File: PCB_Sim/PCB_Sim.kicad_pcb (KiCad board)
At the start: 2 copper layers, 53.3 x 111.8 mm, 12 parts, among them J1 Maneuver_ICS, J2 Loadcell_front_1, J3 Loadcell_front_2, J4 Loadcell_back_1, J5 Loadcell_back_2, J6 Speaker, SW1 SW_DPST_x2, U1 Pico

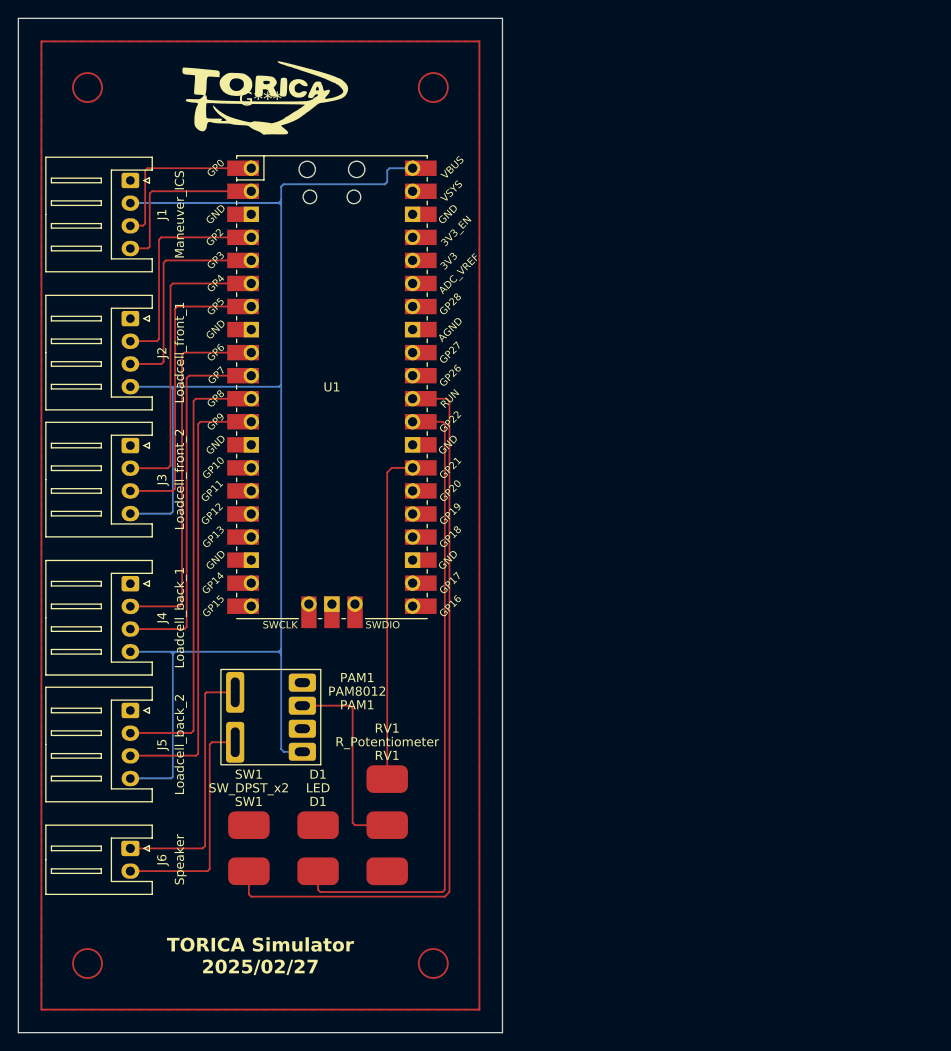
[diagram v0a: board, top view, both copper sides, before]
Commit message: ver.2
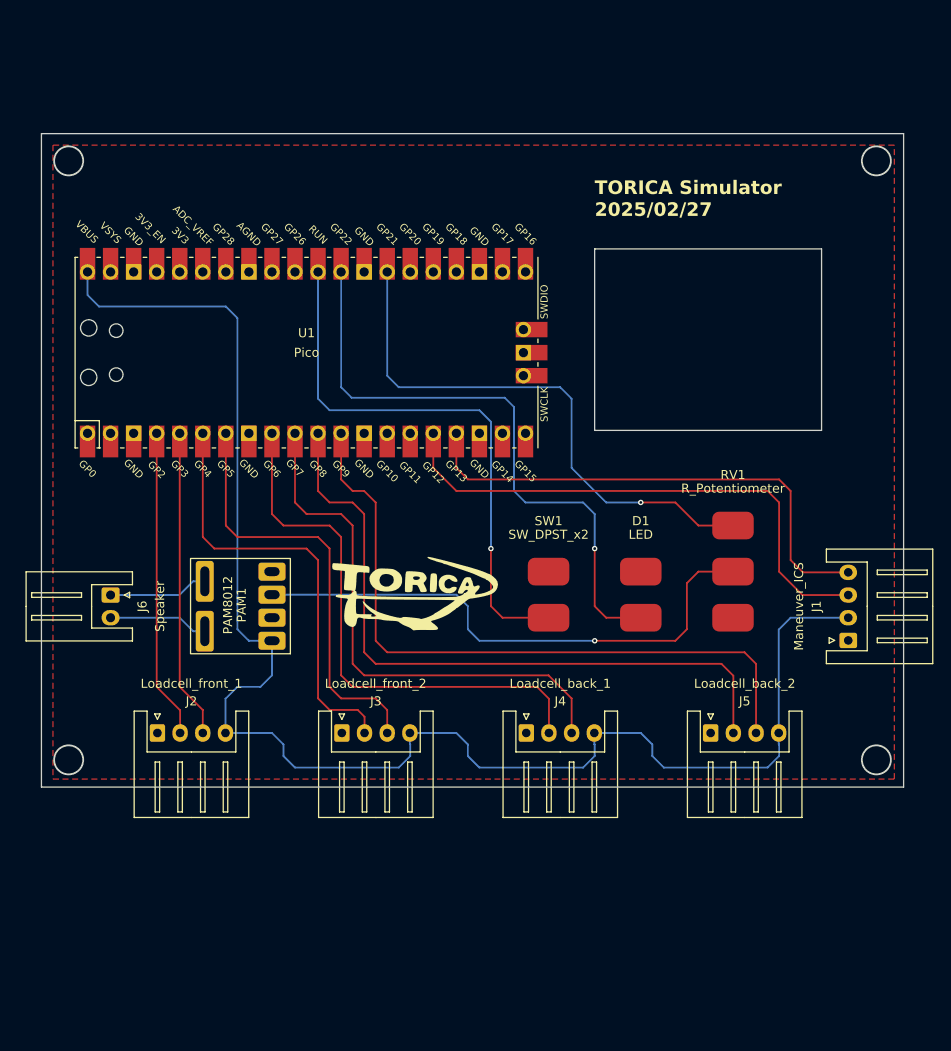
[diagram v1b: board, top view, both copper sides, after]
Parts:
- moved J1 93.9 mm to (190.5, 106.6), turned to 90 degrees
- moved J5 64.0 mm to (175.3, 116.8), turned to 0 degrees
- moved G*** 57.1 mm to (142.2, 101.6)
- moved RV1 47.2 mm to (177.8, 88.9)
- moved J4 46.6 mm to (155.0, 116.8), turned to 0 degrees
- moved J2 45.8 mm to (114.4, 116.8), turned to 0 degrees
- moved D1 45.2 mm to (167.6, 94.0)
- moved SW1 43.3 mm to (157.5, 94.0)
- moved J3 39.3 mm to (134.7, 116.8), turned to 0 degrees
- moved J6 28.0 mm to (109.2, 101.6)
- moved PAM1 12.7 mm to (123.7, 102.8)
- moved U1 4.73 mm to (130.8, 74.9), turned to 90 degrees
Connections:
- U1 pad 1: /PTMR -> unconnected-(U1-GPIO0-Pad1)_1
- U1 pad 16: unconnected-(U1-GPIO12-Pad16) -> /PTMR
- U1 pad 17: unconnected-(U1-GPIO13-Pad17)_1 -> /PRMT
- U1 pad 2: /PRMT -> unconnected-(U1-GPIO1-Pad2)
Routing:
- net /PTMR: track 19.4 -> 59.8 mm
- net Net-(PAM1-in+): track 22.2 -> 60.5 mm, vias 0 -> 1
- net /PRMT: track 19.3 -> 56.2 mm
- net /DAT4: track 49.8 -> 75.8 mm
- net /CLK4: track 49.9 -> 75.8 mm
- net /O_SPK: track 36.8 -> 60.8 mm, vias 0 -> 1
- net /RESET_SW: track 83.2 -> 61.3 mm, vias 0 -> 1
- net /CLK3: track 41.0 -> 60.5 mm
- net /DAT3: track 41.0 -> 59.8 mm
- net /SPK-: track 28.5 -> 11.0 mm
- net /CLK2: track 33.4 -> 48.2 mm
- net /DAT2: track 33.3 -> 47.8 mm
- net /SPK+: track 25.5 -> 11.0 mm
- net /DAT1: track 24.4 -> 34.1 mm
- net /CLK1: track 24.5 -> 34.1 mm
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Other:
- board size 53.3 x 111.8 mm -> 95 x 72 mm
